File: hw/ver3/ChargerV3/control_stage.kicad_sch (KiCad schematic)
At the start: 1 part

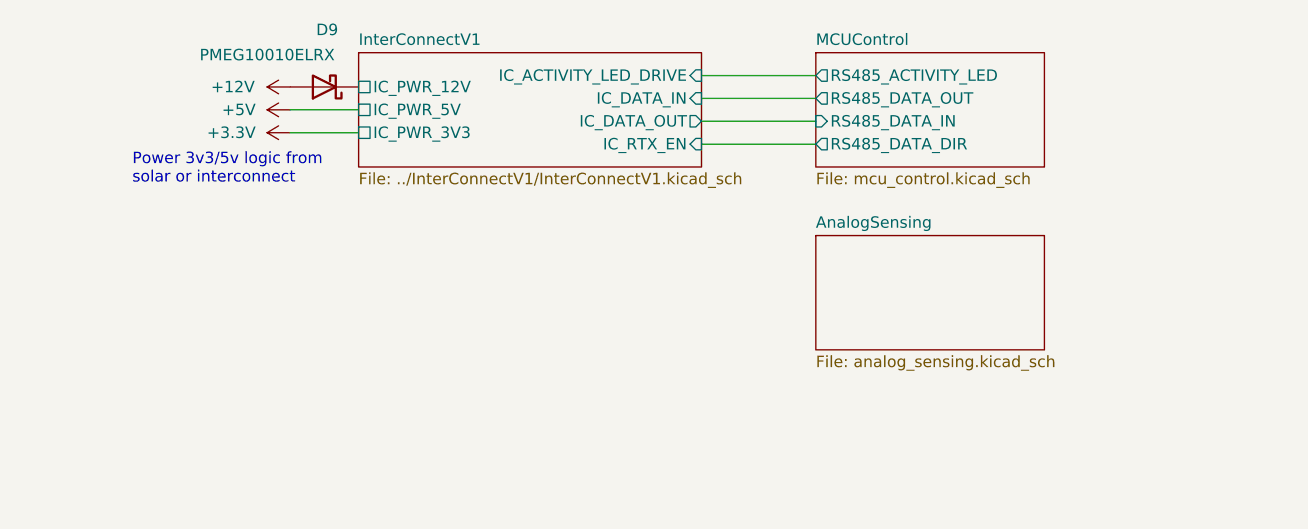
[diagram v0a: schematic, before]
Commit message: Sync board changes from before work started
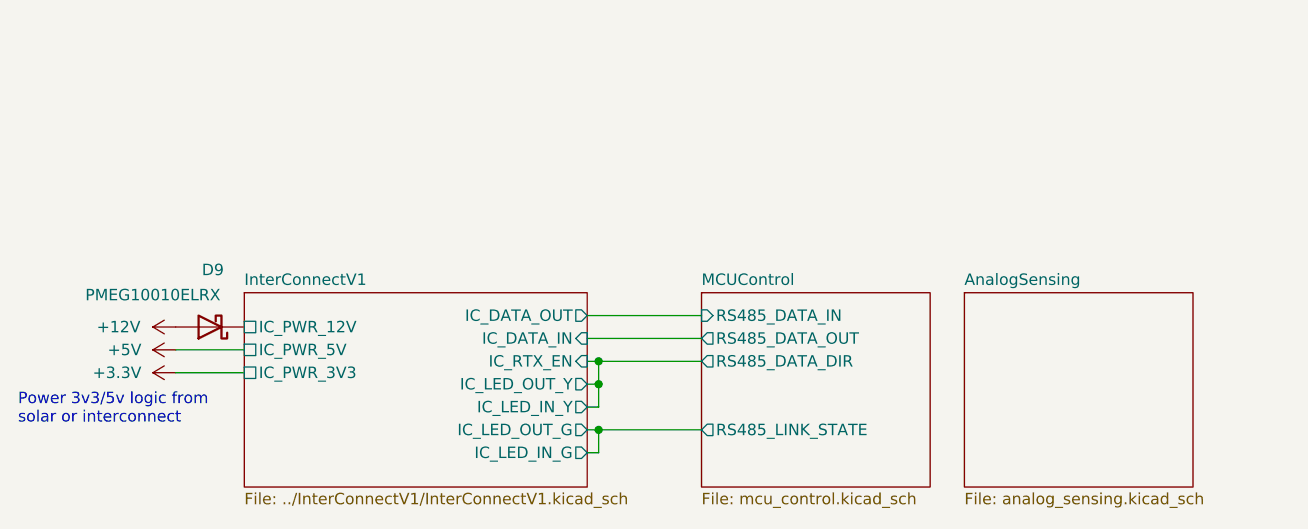
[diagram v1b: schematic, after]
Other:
- sheet InterConnectV1 ports: added IC_LED_IN_G, IC_LED_IN_Y, IC_LED_OUT_G, IC_LED_OUT_Y; removed IC_ACTIVITY_LED_DRIVE
- sheet MCUControl ports: added RS485_LINK_STATE; removed RS485_ACTIVITY_LED
- moved on the sheet: D9
